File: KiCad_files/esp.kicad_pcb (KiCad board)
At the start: 2 copper layers, 100 x 100 mm, 65 parts, among them J1 Conn_01x02_Pin, J2 USB4105-GF-A, J3 Conn_01x16_Pin, Q2 DMP3099L, SW1 SLW-171175-7A-N-D, U1 B3U-1000P, U12 ESP32-S3-MINI-1U, U13 BNO085, U2 1060, U7 LTC4412xS6

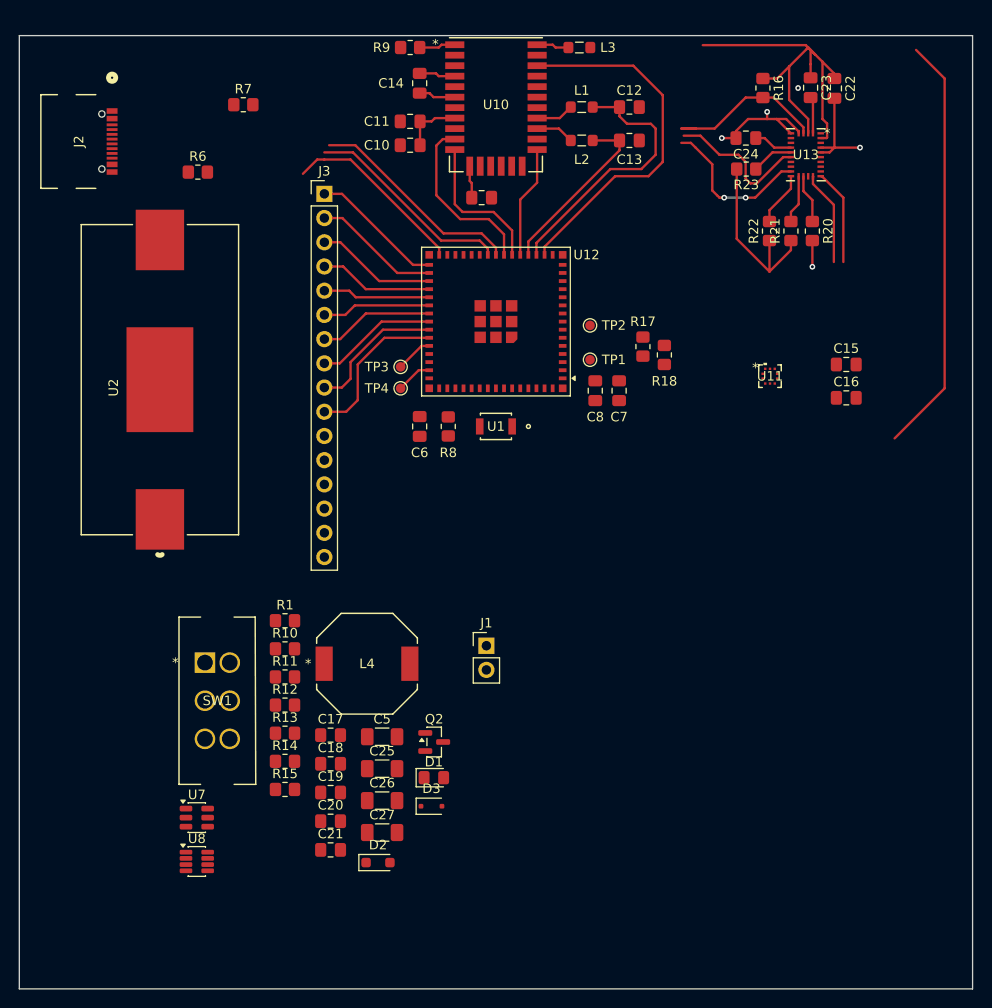
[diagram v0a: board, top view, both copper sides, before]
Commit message: wip
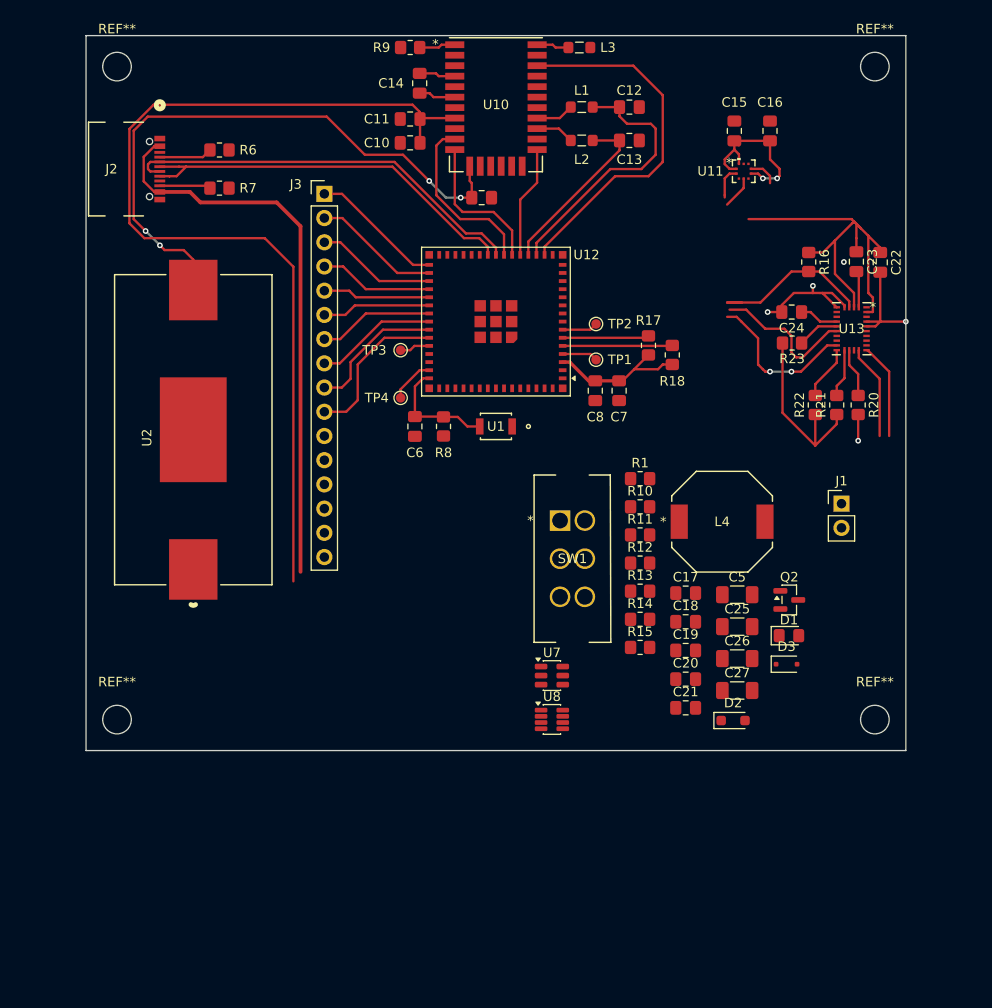
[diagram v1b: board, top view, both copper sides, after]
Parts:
- added REF**: MountingHole_3mm, MountingHole:MountingHole_3mm, F.Cu at (85.2, 28.2)
- added REF**: MountingHole_3mm, MountingHole:MountingHole_3mm, F.Cu at (164.8, 28.2)
- added REF**: MountingHole_3mm, MountingHole:MountingHole_3mm, F.Cu at (85.2, 96.8)
- added REF**: MountingHole_3mm, MountingHole:MountingHole_3mm, F.Cu at (164.8, 96.8)
- moved D1 40.1 mm to (155.7, 87.9)
- moved D3 40.1 mm to (155.5, 90.9)
- moved Q2 40.1 mm to (155.8, 84.2)
- moved C18 40.1 mm to (144.9, 86.5)
- moved C19 40.1 mm to (144.9, 89.5)
- moved C21 40.1 mm to (144.9, 95.5)
- moved C25 40.1 mm to (150.3, 87.0)
- moved C26 40.1 mm to (150.3, 90.3)
- moved D2 40.1 mm to (149.9, 96.8)
- moved J1 40.1 mm to (161.2, 74.1)
- moved L4 40.1 mm to (148.7, 76.0)
- moved R11 40.1 mm to (140.1, 77.4)
- moved R12 40.1 mm to (140.1, 80.3)
- moved R13 40.1 mm to (140.1, 83.3)
- moved U8 40.1 mm to (130.9, 96.7)
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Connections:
- U12 pad 11: /BAROMETER_INT -> unconnected-(U12-IO7-Pad11)
- U12 pad 16: unconnected-(U12-IO12-Pad16) -> /BAROMETER_INT
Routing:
- net +3.3V: track 112.9 -> 196.2 mm, vias 0 -> 2
- net Net-(U10-BV): track 3.39 -> 64.8 mm, vias 0 -> 4
- net /USB_VBUS: track 0.00 -> 59.4 mm
- net /USB_D-: track 22.7 -> 42.9 mm
- net /USB_D+: track 22.0 -> 41.9 mm
- net /BAT_STAT: track 19.5 -> 0.00 mm
- net /I2C_SDA: track 10.1 -> 25.0 mm
- net /I2C_CLK: track 9.93 -> 22.4 mm
- net Net-(U12-EN): track 0.00 -> 12.2 mm
- net Net-(J2-CC1): track 0.00 -> 5.57 mm
- net Net-(J2-CC2): track 0.00 -> 5.37 mm
- net Net-(U12-IO3): track 0.00 -> 3.75 mm
- net Net-(U12-IO0): track 0.00 -> 3.75 mm
- net /BAROMETER_INT: track 0.00 -> 3.06 mm
- net Net-(U12-IO46): track 3.79 -> 4.73 mm
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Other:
- board size 100 x 100 mm -> 86 x 75 mm
